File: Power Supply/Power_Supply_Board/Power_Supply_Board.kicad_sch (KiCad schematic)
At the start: 38 parts, among them SW1 Standby

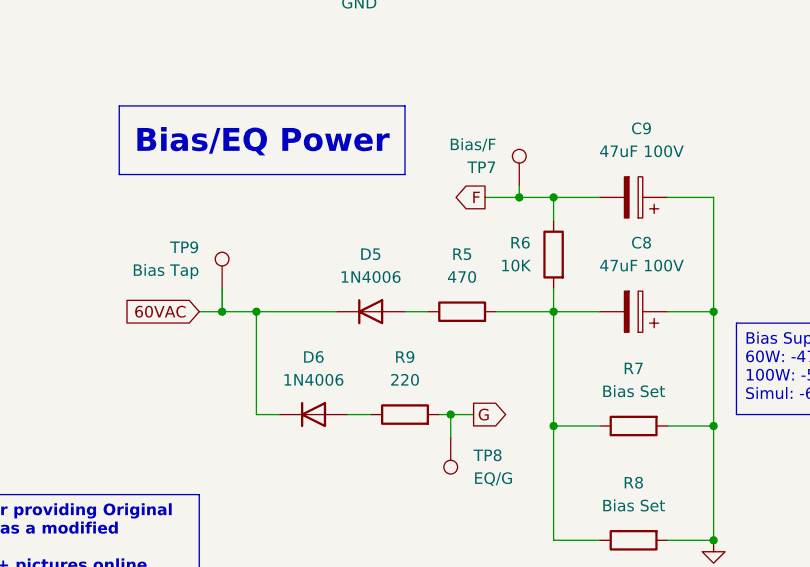
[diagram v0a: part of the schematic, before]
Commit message: Power Supply Board Progress
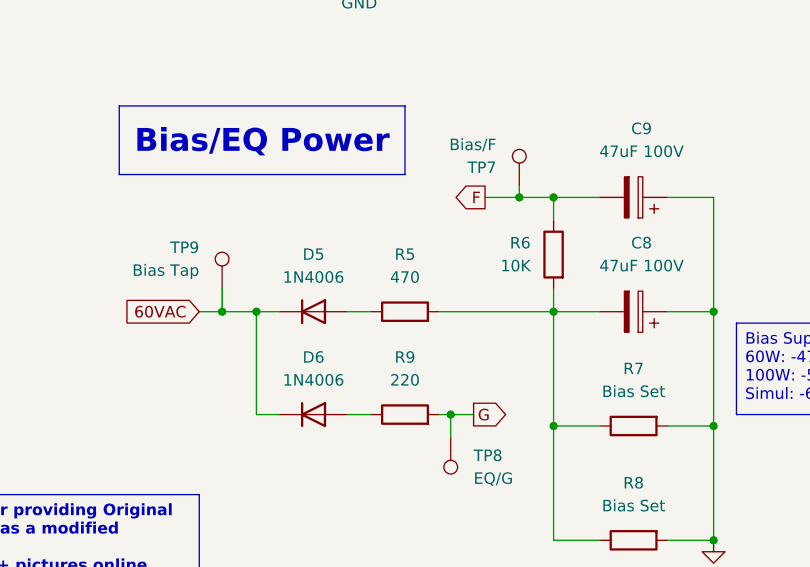
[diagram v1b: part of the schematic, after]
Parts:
- C1, C2, C3, C4: footprint Capacitor_THT:CP_Axial_L30.0mm_D18.0mm_P35.00mm_Horizontal -> Capacitor_THT:CP_Axial_L55.0mm_D26.0mm_P60.00mm_Horizontal
- C5, C6, C7: footprint Capacitor_THT:CP_Axial_L38.0mm_D21.0mm_P44.00mm_Horizontal -> Capacitor_THT:CP_Axial_L42.0mm_D26.0mm_P45.00mm_Horizontal
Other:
- moved on the sheet: D5, R5
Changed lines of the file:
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@@
 	(wire
 		(pts
-			(xy 90.17 152.4) (xy 99.06 152.4)
+			(xy 90.17 152.4) (xy 92.71 152.4)
 		)
 		(stroke
@@
 	(wire
 		(pts
-			(xy 109.22 152.4) (xy 106.68 152.4)
+			(xy 102.87 152.4) (xy 100.33 152.4)
 		)
 		(stroke
@@
 	(wire
 		(pts
-			(xy 116.84 152.4) (xy 123.19 152.4)
+			(xy 110.49 152.4) (xy 123.19 152.4)
 		)
 		(stroke
@@
 			)
 		)
-		(property "Footprint" "Capacitor_THT:CP_Axial_L38.0mm_D21.0mm_P44.00mm_Horizontal"
+		(property "Footprint" "Capacitor_THT:CP_Axial_L42.0mm_D26.0mm_P45.00mm_Horizontal"
 			(at 159.7152 90.17 0)
 			(effects
@@
 			)
 		)
-		(property "Footprint" "Capacitor_THT:CP_Axial_L30.0mm_D18.0mm_P35.00mm_Horizontal"
+		(property "Footprint" "Capacitor_THT:CP_Axial_L55.0mm_D26.0mm_P60.00mm_Horizontal"
 			(at 102.5652 106.68 0)
 			(effects
@@
 			)
 		)
-		(property "Footprint" "Capacitor_THT:CP_Axial_L30.0mm_D18.0mm_P35.00mm_Horizontal"
+		(property "Footprint" "Capacitor_THT:CP_Axial_L55.0mm_D26.0mm_P60.00mm_Horizontal"
 			(at 102.5652 90.17 0)
 			(effects
@@
 			)
 		)
-		(property "Footprint" "Capacitor_THT:CP_Axial_L38.0mm_D21.0mm_P44.00mm_Horizontal"
+		(property "Footprint" "Capacitor_THT:CP_Axial_L42.0mm_D26.0mm_P45.00mm_Horizontal"
 			(at 195.2752 90.17 0)
 			(effects
@@
 	(symbol
 		(lib_id "Diode:1N4006")
-		(at 102.87 152.4 0)
+		(at 96.52 152.4 0)
 		(unit 1)
 		(exclude_from_sim no)
@@
 		(dnp no)
 		(property "Reference" "D5"
-			(at 102.87 146.05 0)
+			(at 96.52 146.05 0)
 			(effects
 				(font
@@
 		)
 		(property "Value" "1N4006"
-			(at 102.87 148.59 0)
+			(at 96.52 148.59 0)
 			(effects
 				(font
@@
 		)
 		(property "Footprint" "Diode_THT:D_DO-41_SOD81_P10.16mm_Horizontal"
-			(at 102.87 156.845 0)
+			(at 96.52 156.845 0)
 			(effects
 				(font
@@
 		)
 		(property "Datasheet" "http://www.vishay.com/docs/88503/1n4001.pdf"
-			(at 102.87 152.4 0)
+			(at 96.52 152.4 0)
 			(effects
 				(font
@@
 		)
 		(property "Description" "800V 1A General Purpose Rectifier Diode, DO-41"
-			(at 102.87 152.4 0)
+			(at 96.52 152.4 0)
 			(effects
 				(font
@@
 		)
 		(property "Sim.Device" "D"
-			(at 102.87 152.4 0)
+			(at 96.52 152.4 0)
 			(effects
 				(font
@@
 		)
 		(property "Sim.Pins" "1=K 2=A"
-			(at 102.87 152.4 0)
+			(at 96.52 152.4 0)
 			(effects
 				(font
@@
 			)
 		)
-		(property "Footprint" "Capacitor_THT:CP_Axial_L38.0mm_D21.0mm_P44.00mm_Horizontal"
+		(property "Footprint" "Capacitor_THT:CP_Axial_L42.0mm_D26.0mm_P45.00mm_Horizontal"
 			(at 177.4952 90.17 0)
 			(effects
@@
 			)
 		)
-		(property "Footprint" "Capacitor_THT:CP_Axial_L30.0mm_D18.0mm_P35.00mm_Horizontal"
+		(property "Footprint" "Capacitor_THT:CP_Axial_L55.0mm_D26.0mm_P60.00mm_Horizontal"
 			(at 122.8852 90.17 0)
 			(effects
@@
 			)
 		)
-		(property "Footprint" "Capacitor_THT:CP_Axial_L30.0mm_D18.0mm_P35.00mm_Horizontal"
+		(property "Footprint" "Capacitor_THT:CP_Axial_L55.0mm_D26.0mm_P60.00mm_Horizontal"
 			(at 122.8852 106.68 0)
 			(effects
@@
 	(symbol
 		(lib_id "Device:R")
-		(at 113.03 152.4 90)
+		(at 106.68 152.4 90)
 		(unit 1)
 		(exclude_from_sim no)
@@
 		(fields_autoplaced yes)
 		(property "Reference" "R5"
-			(at 113.03 146.05 90)
+			(at 106.68 146.05 90)
 			(effects
 				(font
@@
 		)
 		(property "Value" "470"
-			(at 113.03 148.59 90)
+			(at 106.68 148.59 90)
 			(effects
 				(font
@@
 		)
 		(property "Footprint" "Resistor_THT:R_Axial_DIN0516_L15.5mm_D5.0mm_P20.32mm_Horizontal"
-			(at 113.03 154.178 90)
+			(at 106.68 154.178 90)
 			(effects
 				(font
@@
 		)
 		(property "Datasheet" "~"
-			(at 113.03 152.4 0)
+			(at 106.68 152.4 0)
 			(effects
 				(font
@@
 		)
 		(property "Description" "Resistor"
-			(at 113.03 152.4 0)
+			(at 106.68 152.4 0)
 			(effects
 				(font
